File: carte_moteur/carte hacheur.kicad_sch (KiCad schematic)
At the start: 30 parts, among them IC1 VNH7100BASTR, IC2 VNH7100BASTR, J1 Conn_01x02_Pin, J2 Conn_01x02_Pin, J3 Conn_01x02_Pin, J4 RJ11, Q1 PMOS, U2 MCP2562-E-P, U3 MCP2515-xSO

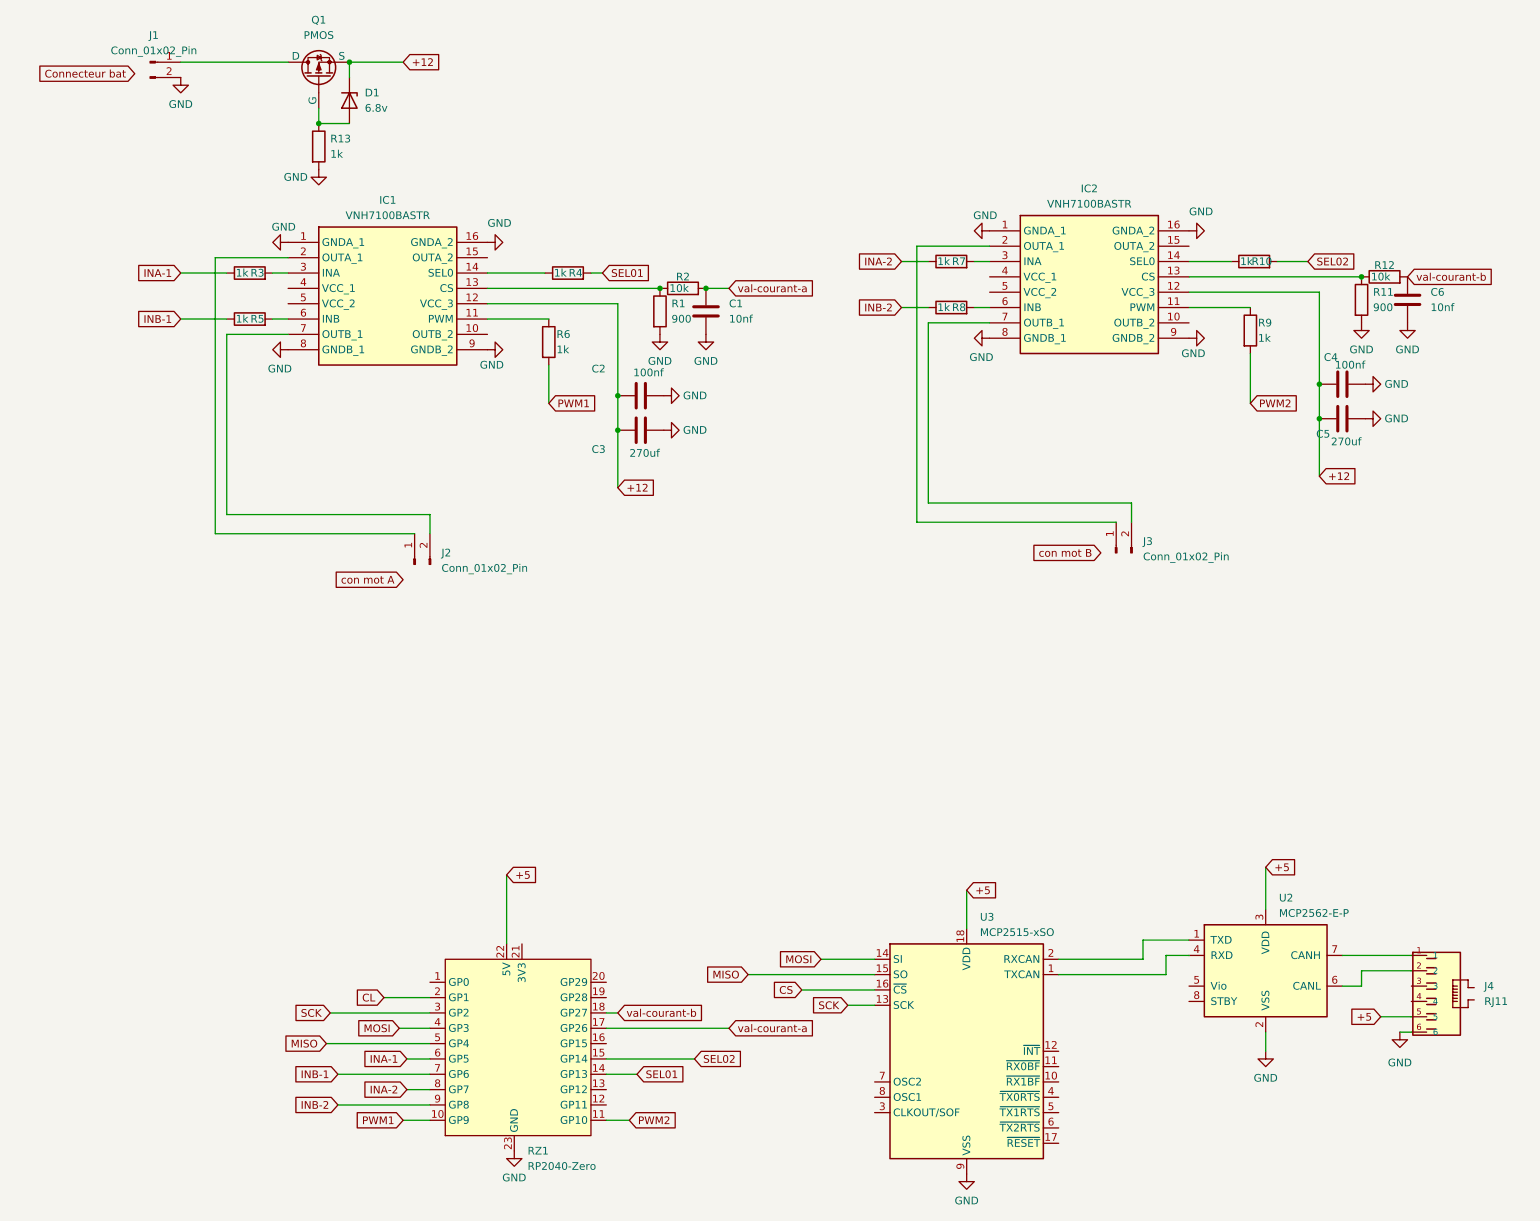
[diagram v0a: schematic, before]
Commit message: carte bat
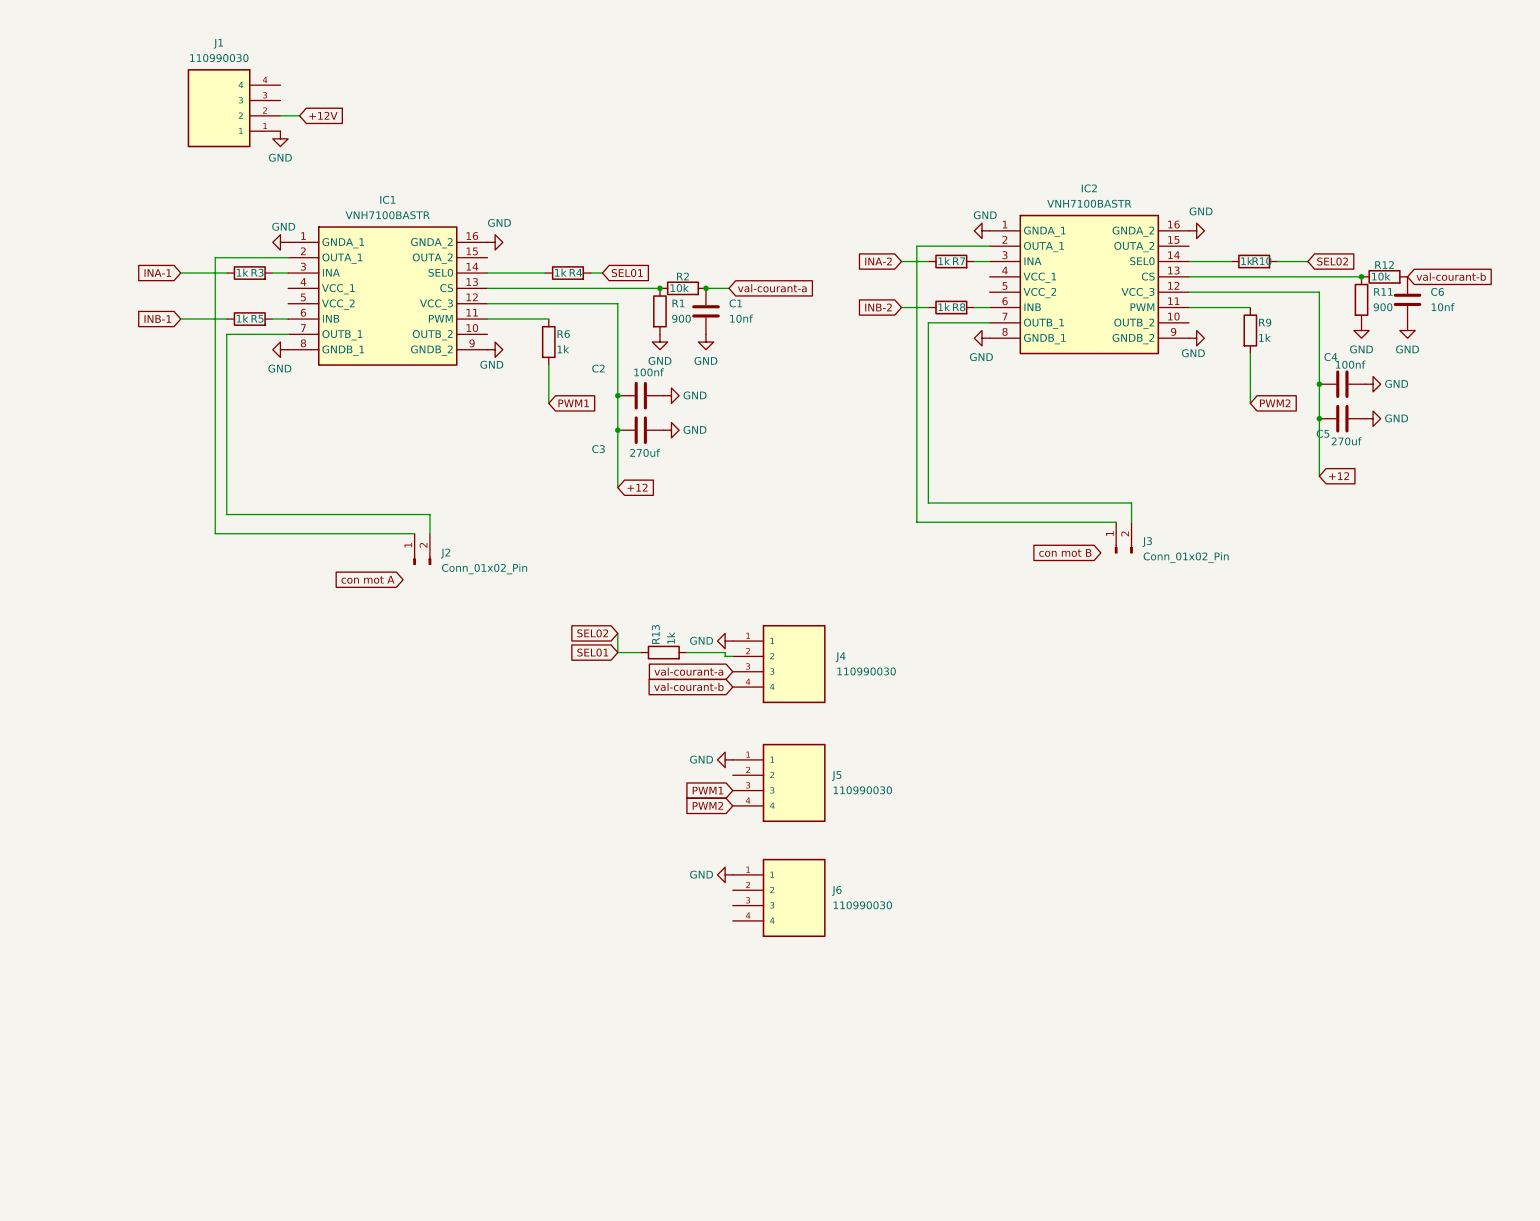
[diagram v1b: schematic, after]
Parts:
- removed D1: 6.8v, symbol Device:D_Zener
- removed J1: Conn_01x02_Pin, symbol Connector:Conn_01x02_Pin
- removed J4: RJ11, symbol RJ11:RJ11
- removed Q1: PMOS, symbol Simulation_SPICE:PMOS
- removed RZ1: RP2040-Zero, symbol rp2040-zero:RP2040-Zero
- removed U2: MCP2562-E-P, Package_DIP:DIP-8_W7.62mm, symbol Interface_CAN_LIN:MCP2562-E-P
- removed U3: MCP2515-xSO, Package_SO:SOIC-18W_7.5x11.6mm_P1.27mm, symbol Interface_CAN_LIN:MCP2515-xSO
- added J1, J4, J5, J6: 110990030, symbol 110990030:110990030
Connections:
- net SEL02 is gone; now on net SEL01: R10.2
- net GND: now also J1.1, J4.1, J5.1, J6.1; no longer R13.2
- net PWM1: now also J5.3
- net PWM2: now also J5.4
- net SEL01: now also R13.1
- net val-courant-a: now also J4.3
- net val-courant-b: now also J4.4
- new net: J4.2, R13.2
- new net +12V: J1.2
